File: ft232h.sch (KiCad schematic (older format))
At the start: 15 parts, among them U2 93LCxxB, U3 FT232H, Y2 Crystal_GND24

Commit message: schematics for expansion slots and memory
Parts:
- R29: footprint (none) -> Resistor_SMD:R_0603_1608Metric
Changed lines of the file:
@@
 $Descr A4 11693 8268
 encoding utf-8
-Sheet 3 5
+Sheet 5 10
 Title ""
 Date "2019-03-16"
@@
 F 0 "R4" V 4254 5300 50  0000 C CNN
 F 1 "R_Small" V 4345 5300 50  0000 C CNN
-F 2 "" H 4450 5300 50  0001 C CNN
+F 2 "Resistor_SMD:R_0603_1608Metric" H 4450 5300 50  0001 C CNN
 F 3 "~" H 4450 5300 50  0001 C CNN
 	1    4450 5300

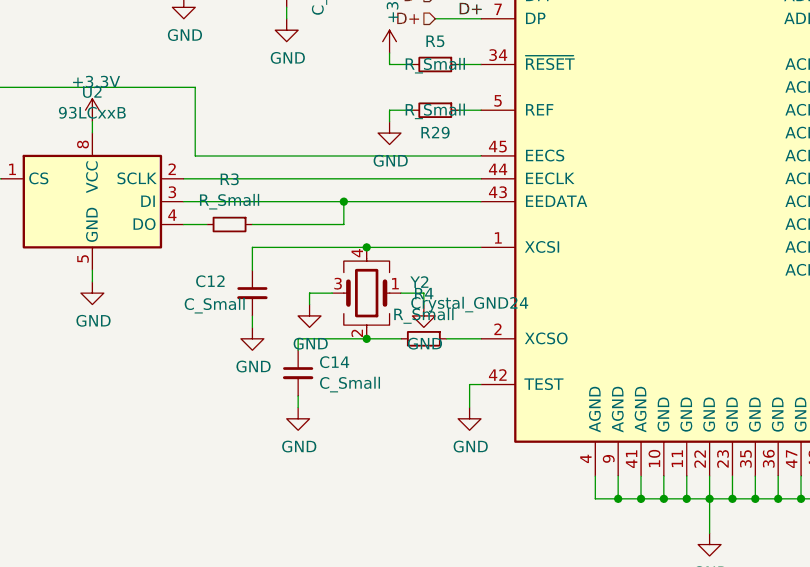
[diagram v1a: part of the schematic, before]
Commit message: almost done with draft 1 of layout
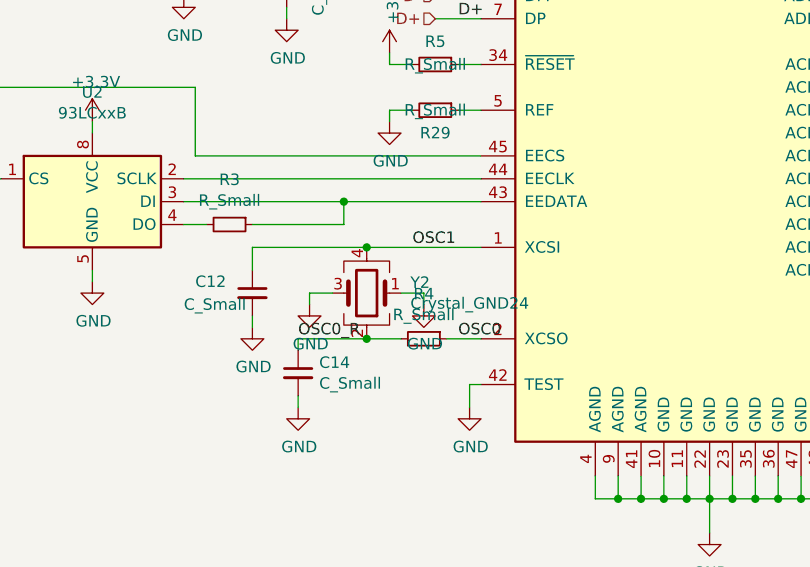
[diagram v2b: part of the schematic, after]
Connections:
- net OSC1: now reaches C12.1, U3.1 (XCSI), Y2.4
- net OSC0: now reaches R29.1, U3.2 (XCSO)
- net OSC0_R: now reaches C14.1, R29.2, Y2.2
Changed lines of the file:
@@
 Wire Wire Line
 	4350 5100 4450 5100
+Text Label 4400 4900 0    50   ~ 0
+OSC1
+Text Label 4600 5300 0    50   ~ 0
+OSC0
+Text Label 3900 5300 0    50   ~ 0
+OSC0_R
 $EndSCHEMATC
